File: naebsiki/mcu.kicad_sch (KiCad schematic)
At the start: 15 parts, among them P1 SWD, U1 STM32F405RGT6, X1 8MHz 10ppm (X50328MSB2GI)

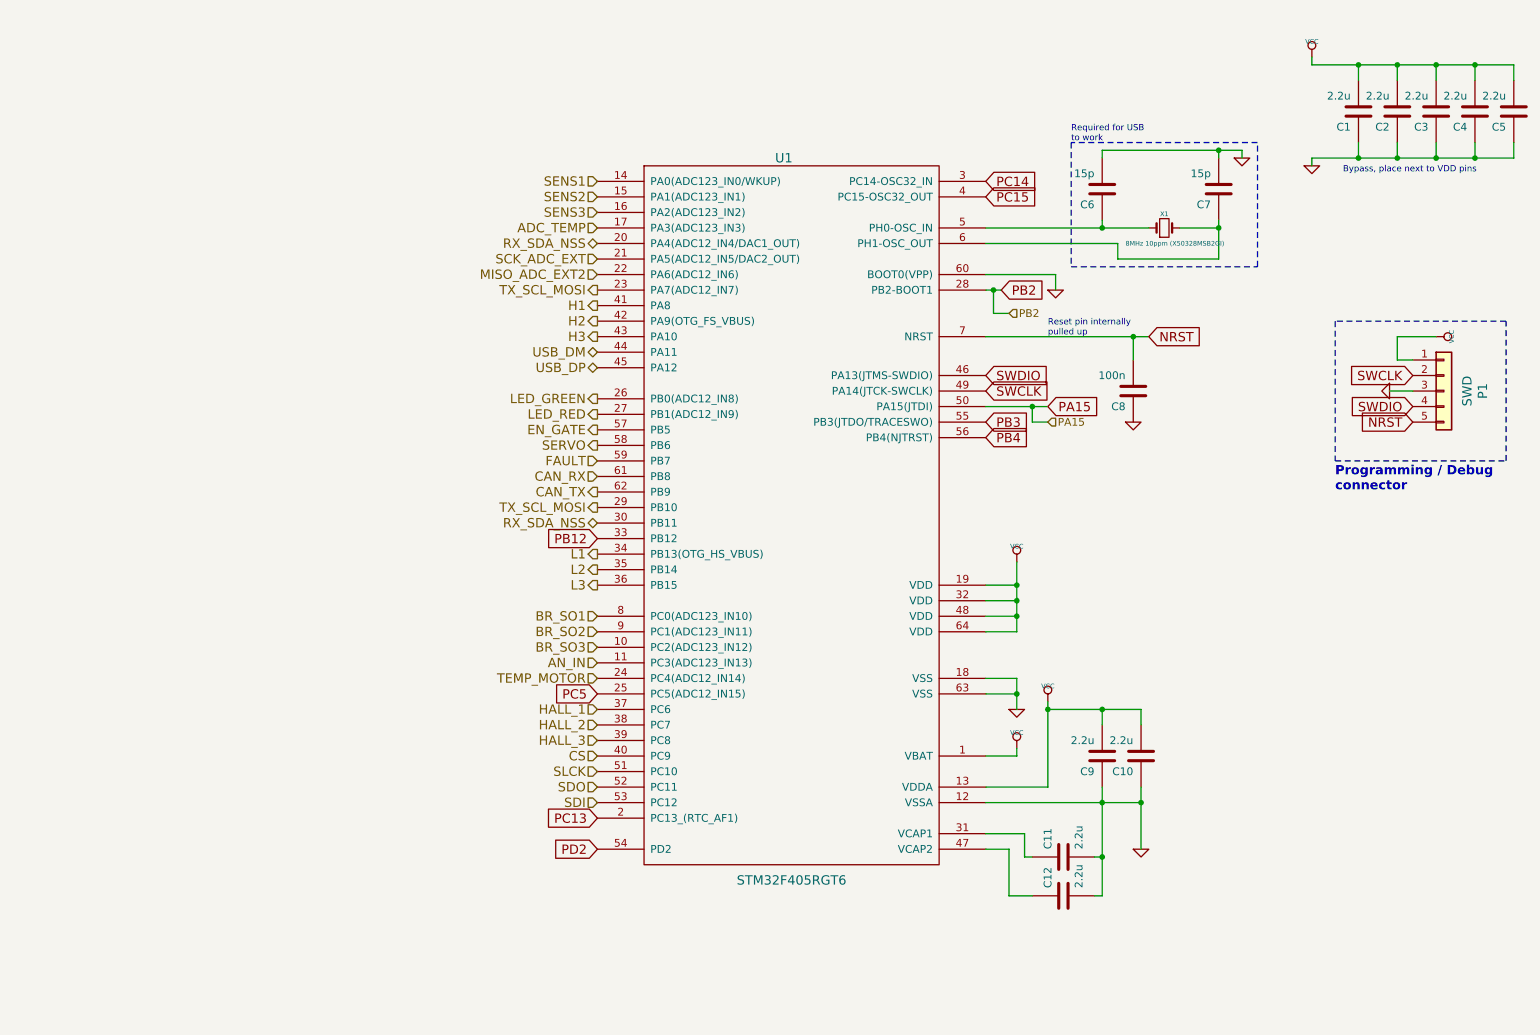
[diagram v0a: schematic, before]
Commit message: final
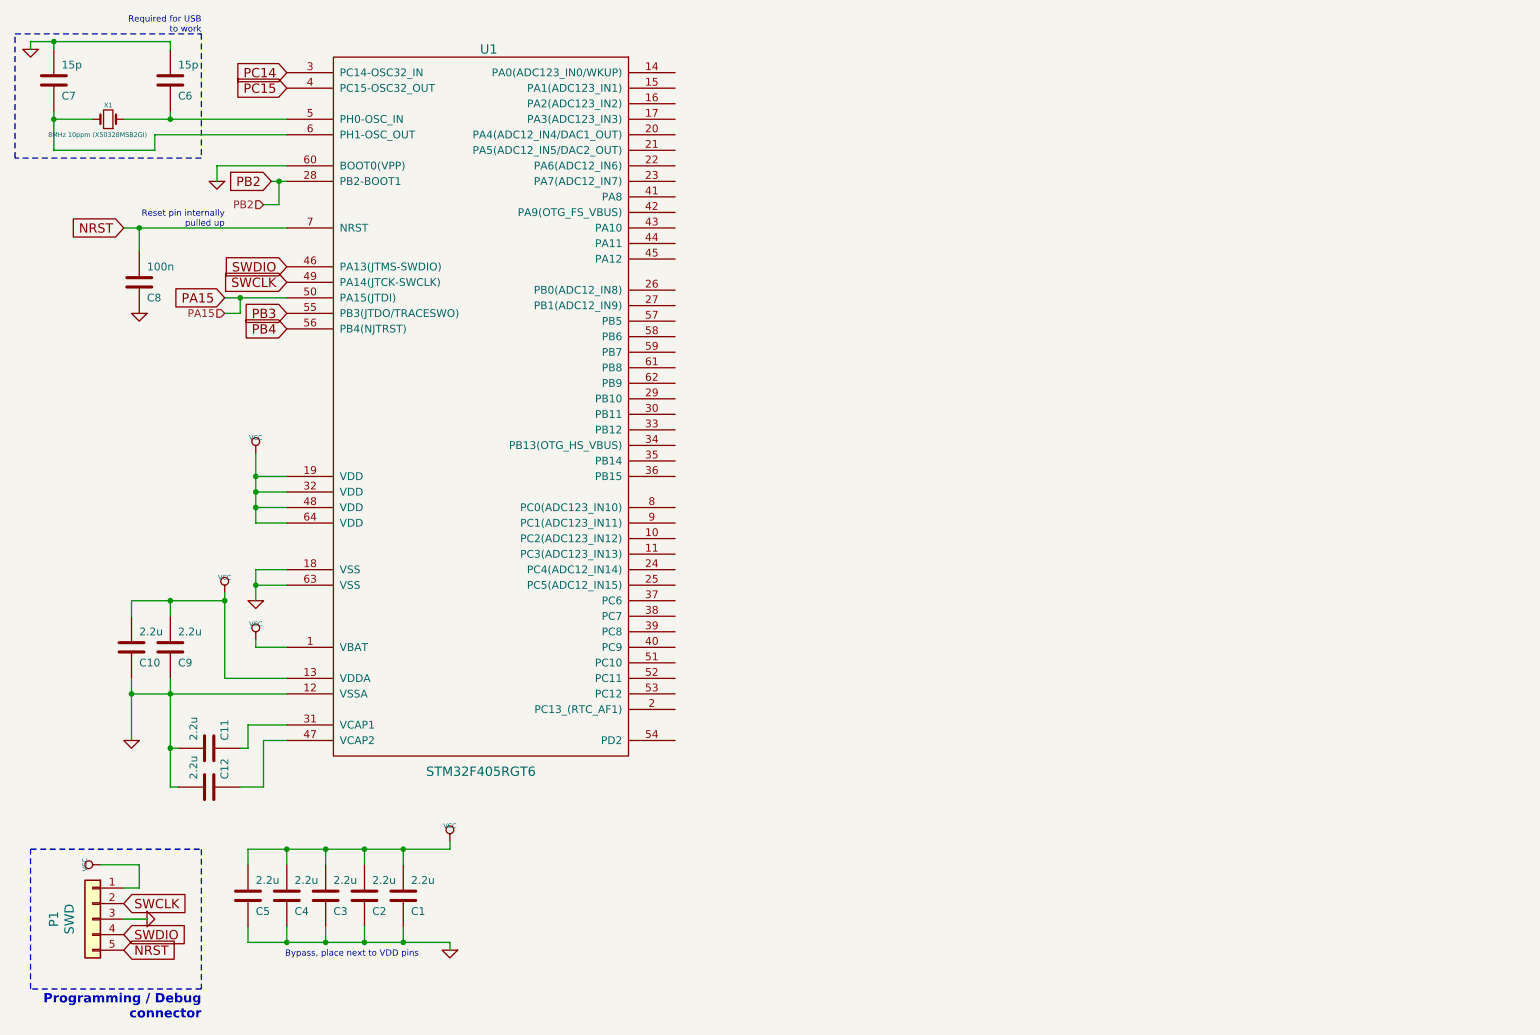
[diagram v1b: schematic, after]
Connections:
- net ADC_TEMP: no longer names the net of U1.17 (PA3(ADC123_IN3))
- net AN_IN: no longer names the net of U1.11 (PC3(ADC123_IN13))
- net BR_SO1: no longer names the net of U1.8 (PC0(ADC123_IN10))
- net BR_SO2: no longer names the net of U1.9 (PC1(ADC123_IN11))
- net BR_SO3: no longer names the net of U1.10 (PC2(ADC123_IN12))
- net CAN_RX: no longer names the net of U1.61 (PB8)
- net CAN_TX: no longer names the net of U1.62 (PB9)
- net CS: no longer names the net of U1.40 (PC9)
- net EN_GATE: no longer names the net of U1.57 (PB5)
- net FAULT: no longer names the net of U1.59 (PB7)
- net H1: no longer names the net of U1.41 (PA8)
- net H2: no longer names the net of U1.42 (PA9(OTG_FS_VBUS))
- net H3: no longer names the net of U1.43 (PA10)
- net HALL_1: no longer names the net of U1.37 (PC6)
- net HALL_2: no longer names the net of U1.38 (PC7)
- net HALL_3: no longer names the net of U1.39 (PC8)
- net L1: no longer names the net of U1.34 (PB13(OTG_HS_VBUS))
- net L2: no longer names the net of U1.35 (PB14)
- net L3: no longer names the net of U1.36 (PB15)
- net LED_GREEN: no longer names the net of U1.26 (PB0(ADC12_IN8))
- net LED_RED: no longer names the net of U1.27 (PB1(ADC12_IN9))
- net MISO_ADC_EXT2: no longer names the net of U1.22 (PA6(ADC12_IN6))
- net PB12: no longer names the net of U1.33 (PB12)
- net PC13: no longer names the net of U1.2 (PC13_(RTC_AF1))
- net PC5: no longer names the net of U1.25 (PC5(ADC12_IN15))
- net PD2: no longer names the net of U1.54 (PD2)
- net RX_SDA_NSS: no longer names the net of U1.20 (PA4(ADC12_IN4/DAC1_OUT))
- net RX_SDA_NSS: no longer U1.30 (PB11)
- net SCK_ADC_EXT: no longer names the net of U1.21 (PA5(ADC12_IN5/DAC2_OUT))
- net SDI: no longer names the net of U1.53 (PC12)
- net SDO: no longer names the net of U1.52 (PC11)
- net SENS1: no longer names the net of U1.14 (PA0(ADC123_IN0/WKUP))
- net SENS2: no longer names the net of U1.15 (PA1(ADC123_IN1))
- net SENS3: no longer names the net of U1.16 (PA2(ADC123_IN2))
- net SERVO: no longer names the net of U1.58 (PB6)
- net SLCK: no longer names the net of U1.51 (PC10)
- net TEMP_MOTOR: no longer names the net of U1.24 (PC4(ADC12_IN14))
- net TX_SCL_MOSI: no longer names the net of U1.23 (PA7(ADC12_IN7))
- net TX_SCL_MOSI: no longer U1.29 (PB10)
- net USB_DM: no longer names the net of U1.44 (PA11)
- net USB_DP: no longer names the net of U1.45 (PA12)
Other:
- moved on the sheet: C1, C10, C11, C12, C2, C3, C4, C5, C6, C7, C8, C9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
